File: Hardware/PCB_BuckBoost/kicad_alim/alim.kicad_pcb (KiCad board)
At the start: 2 copper layers, 36 parts, among them J1 Conn_01x02, J2 Conn_01x02, J3 Conn_01x02, J4 Conn_01x02, U1 MIC3172YM, U2 MIC3172YM

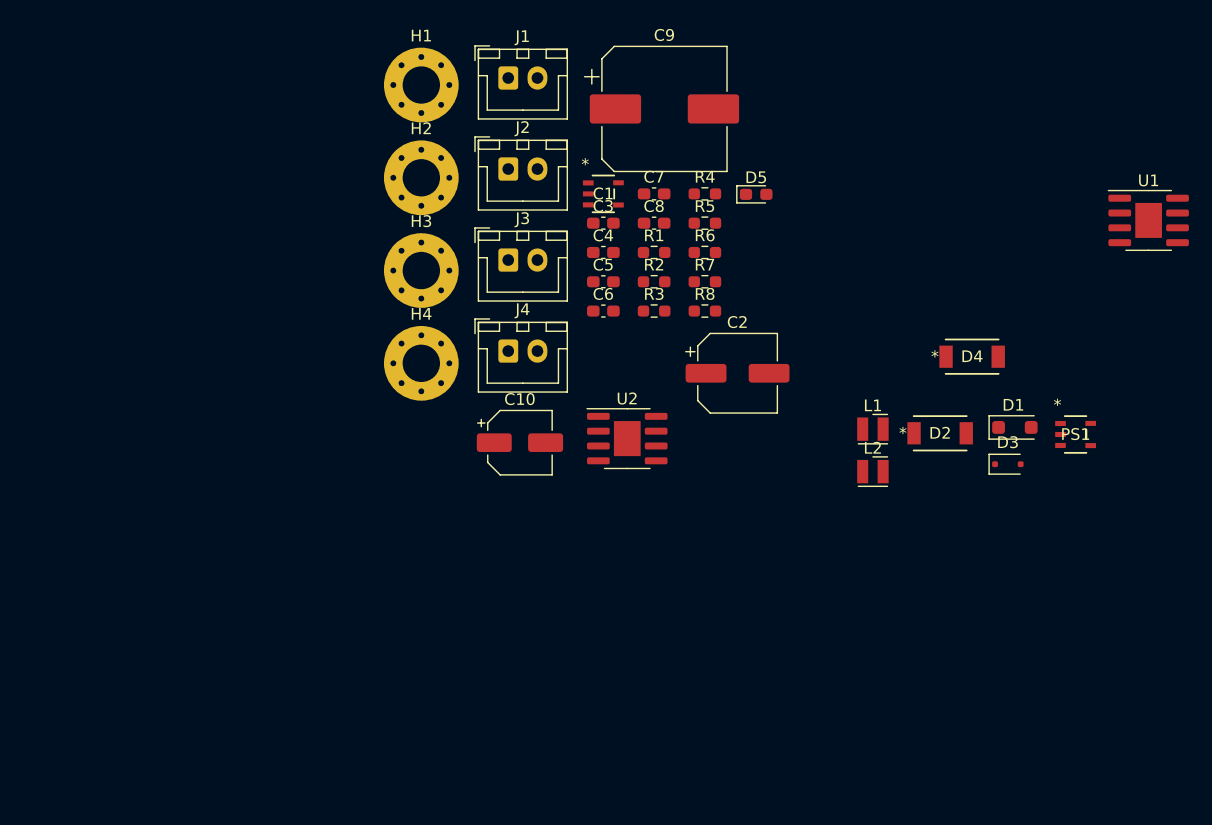
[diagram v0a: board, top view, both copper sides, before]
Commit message: pcb presque terminé (3 erreurs)
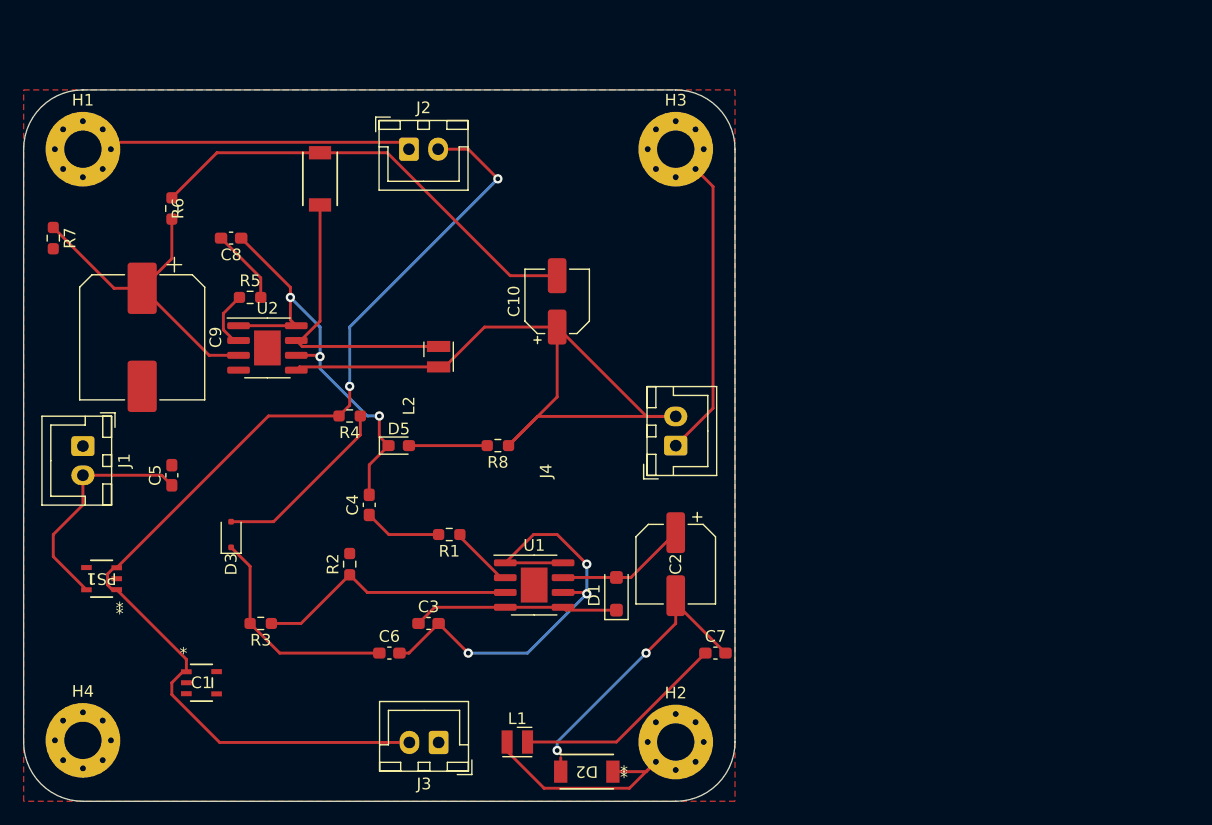
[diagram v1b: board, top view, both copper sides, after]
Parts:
- moved PS1 84.4 mm to (77.8, 87.6), turned to 180 degrees
- moved D3 66.8 mm to (88.9, 83.8), turned to 90 degrees
- moved U1 61.2 mm to (114.9, 88.2)
- moved D4 57.9 mm to (96.5, 53.3), turned to -90 degrees
- moved R7 56.0 mm to (73.7, 58.4), turned to -90 degrees
- moved C1 54.2 mm to (86.4, 96.5)
- moved H2 53.0 mm to (127.0, 101.6)
- moved C9 48.8 mm to (81.3, 66.9), turned to -90 degrees
- moved J1 48.2 mm to (76.2, 76.2), turned to -90 degrees
- moved R6 45.8 mm to (83.8, 55.9), turned to -90 degrees
- moved H4 43.4 mm to (76.2, 101.5)
- moved R3 43.0 mm to (91.4, 91.4), turned to 180 degrees
- moved D2 41.9 mm to (119.4, 104.1), turned to 180 degrees
- moved J3 41.8 mm to (106.7, 101.6), turned to 180 degrees
- moved L1 40.6 mm to (113.4, 101.6)
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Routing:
- net GND: track 0.00 -> 158.3 mm, vias 0 -> 6
- net +5V: track 0.00 -> 112.1 mm, vias 0 -> 2
- net +15V: track 0.00 -> 75.7 mm
- net Routeur: track 0.00 -> 39.0 mm
- net Net-(U2-FB): track 0.00 -> 27.4 mm
- net Net-(D2-A): track 0.00 -> 25.8 mm, vias 0 -> 2
- net Net-(D4-A): track 0.00 -> 25.1 mm
- net Net-(U1-FB): track 0.00 -> 22.4 mm
- net +3.3V: track 0.00 -> 20.0 mm
- net Net-(D3-K): track 0.00 -> 19.3 mm
- net Net-(D1-K): track 0.00 -> 17.6 mm
- net Net-(D3-A): track 0.00 -> 15.8 mm
- net Net-(D5-A): track 0.00 -> 6.71 mm
- net Net-(C4-Pad1): track 0.00 -> 6.64 mm
- net Net-(C8-Pad2): track 0.00 -> 6.49 mm
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- added copper zone on F.Cu, net GND
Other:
- board outline added: 61 x 61 mm
